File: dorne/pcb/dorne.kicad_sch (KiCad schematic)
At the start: 147 parts, among them J1 MJ-4PP-9, J2 OLED, J3 MJ-4PP-9, J4 OLED, SW1 SW_PUSH, SW10 SW_PUSH, SW11 SW_PUSH, SW12 SW_PUSH, SW13 SW_PUSH, SW14 SW_PUSH, SW15 SW_PUSH, SW16 SW_PUSH, SW17 SW_PUSH, SW18 SW_PUSH, SW19 SW_PUSH, SW2 SW_PUSH, SW20 SW_PUSH, SW21 SW_PUSH, SW22 SW_PUSH, SW23 SW_PUSH, SW24 SW_PUSH, SW25 SW_PUSH, SW26 SW_PUSH, SW27 SW_PUSH, SW28 SW_PUSH, SW29 SW_PUSH, SW3 SW_PUSH, SW30 SW_PUSH, SW31 SW_PUSH, SW32 SW_PUSH, SW33 SW_PUSH, SW34 SW_PUSH, SW35 SW_PUSH, SW36 SW_PUSH, SW37 SW_PUSH, SW38 SW_PUSH, SW39 SW_PUSH, SW4 SW_PUSH, SW40 SW_PUSH, SW41 SW_PUSH, SW42 SW_PUSH, SW5 SW_PUSH, SW6 SW_PUSH, SW7 SW_PUSH, SW8 SW_PUSH, SW9 SW_PUSH, U1 ProMicro, U1 nice_nano, U2 ProMicro

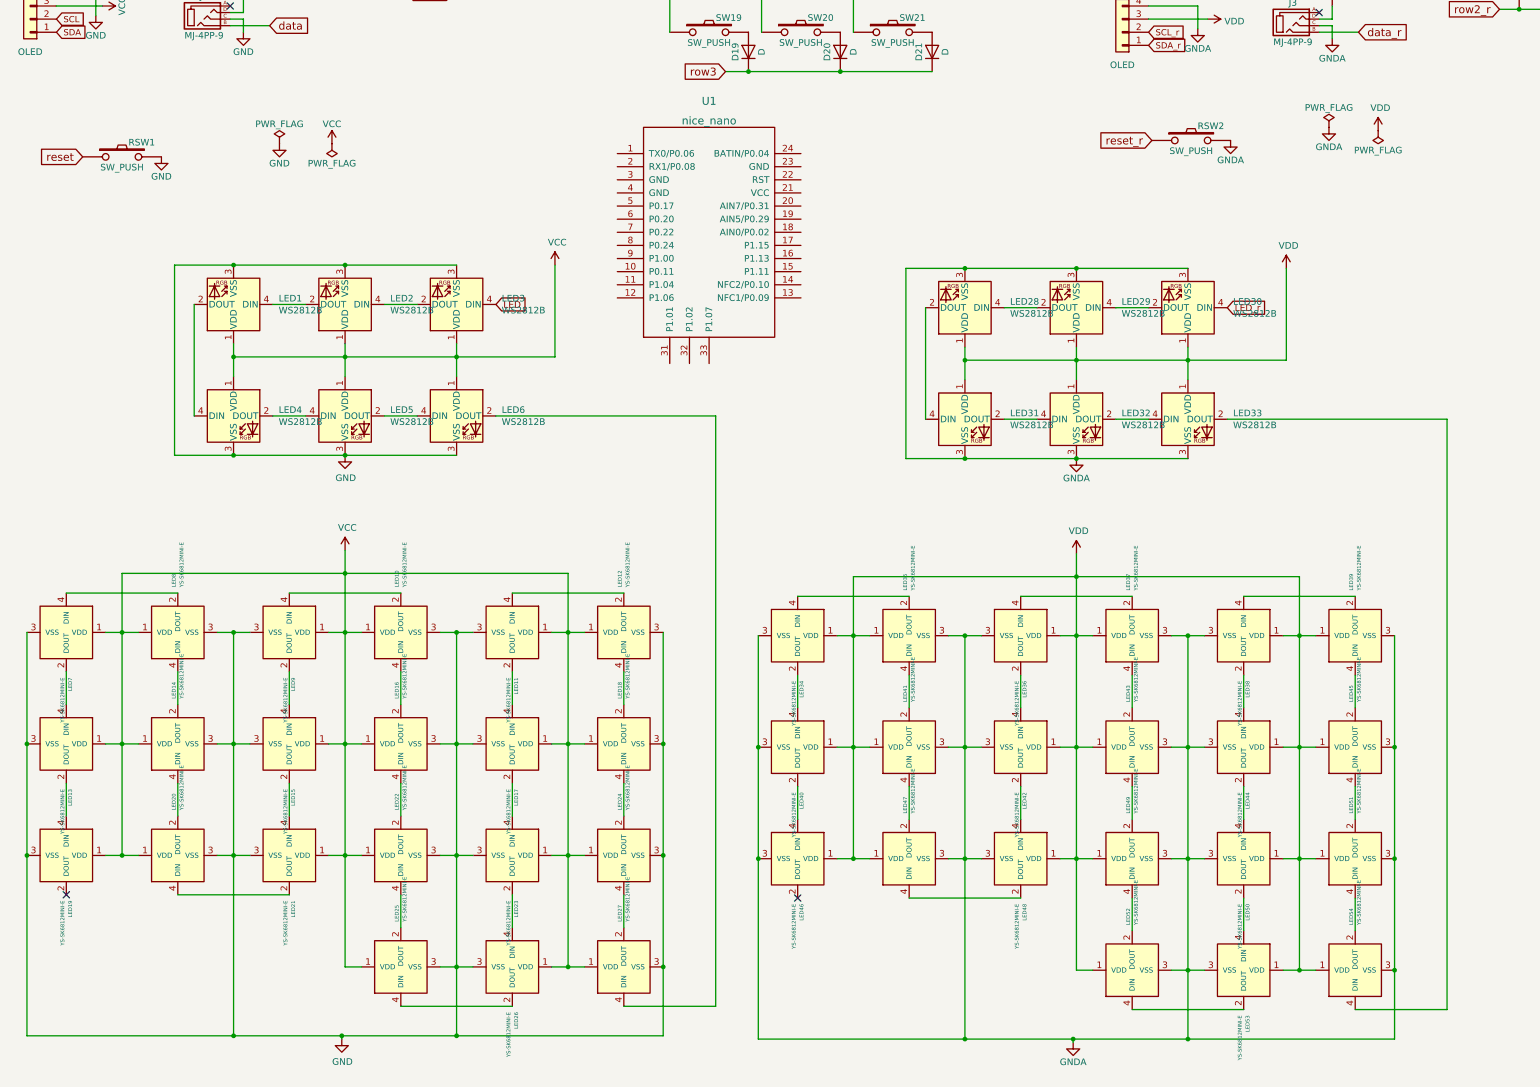
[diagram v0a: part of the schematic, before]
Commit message: RM LEDs
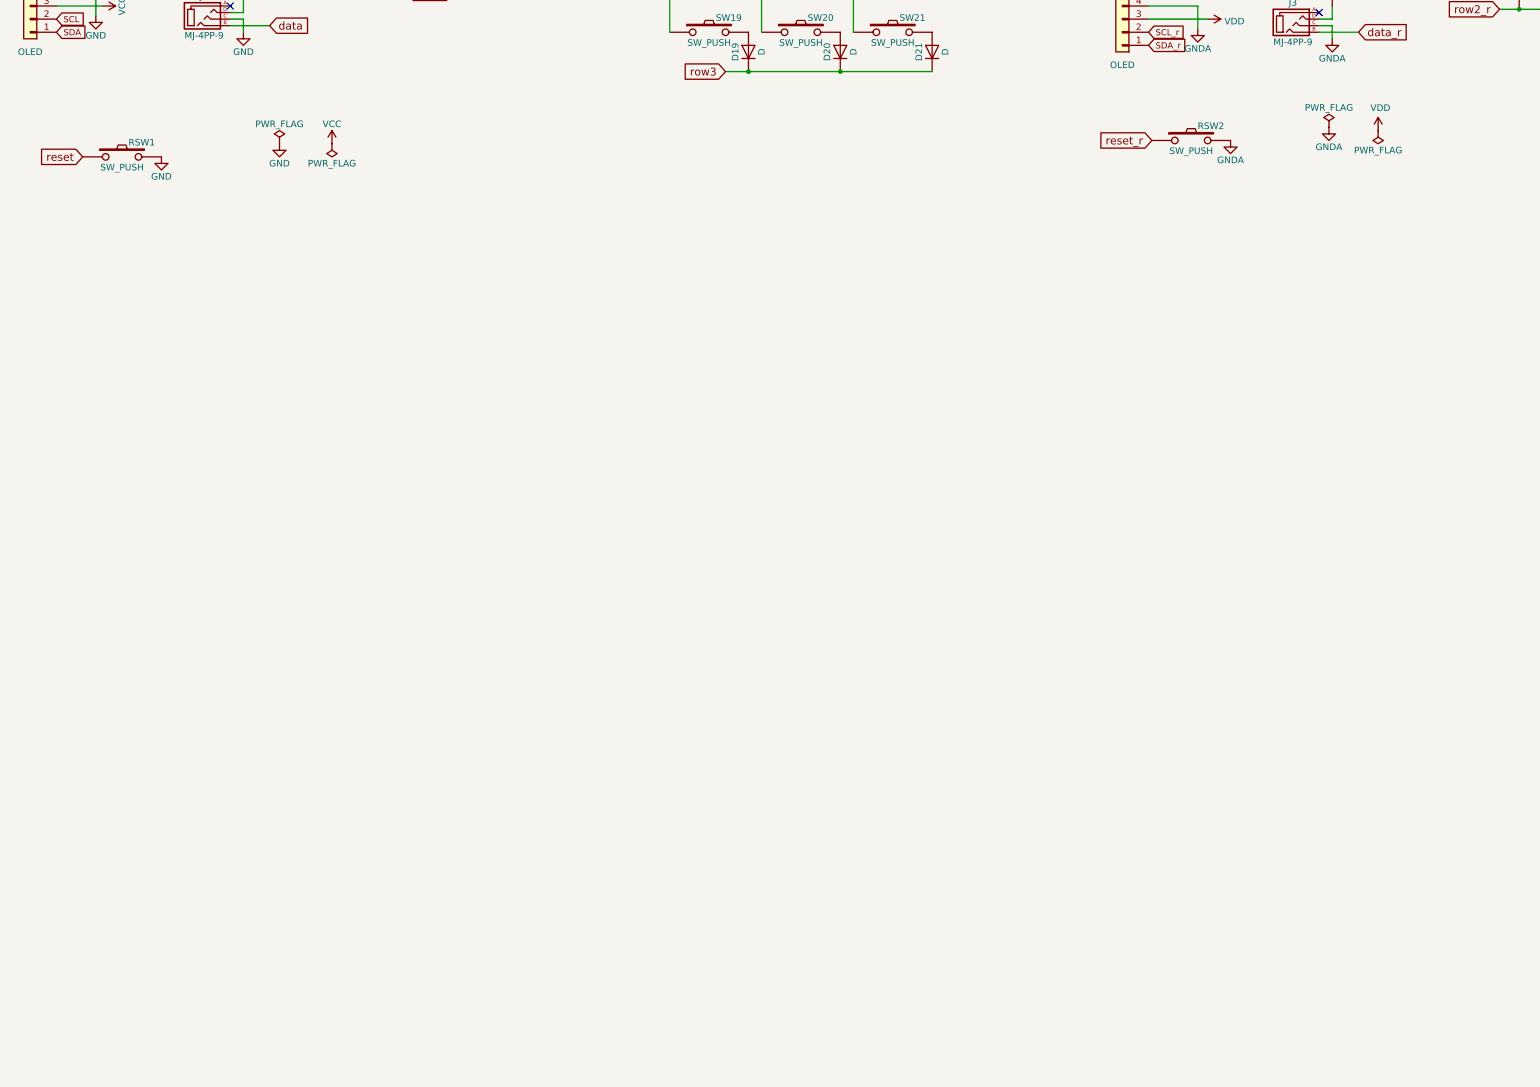
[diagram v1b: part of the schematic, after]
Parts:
- removed LED1, LED2, LED28, LED29, LED3, LED30, LED31, LED32, LED33, LED4, LED5, LED6: WS2812B, LED_SMD:LED_WS2812B_PLCC4_5.0x5.0mm_P3.2mm, symbol LED:WS2812B
- removed LED10, LED11, LED12, LED13, LED14, LED15, LED16, LED17, LED18, LED19, LED20, LED21, LED22, LED23, LED24, LED25, LED26, LED27, LED34, LED35, LED36, LED37, LED38, LED39, LED40, LED41, LED42, LED43, LED44, LED45, LED46, LED47, LED48, LED49, LED50, LED51, LED52, LED53, LED54, LED7, LED8, LED9: YS-SK6812MINI-E, kbd:YS-SK6812MINI-E, symbol kbd:YS-SK6812MINI-E
- removed U1: nice_nano, symbol nice:nice_nano
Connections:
- no-connect marks 14 -> 12
